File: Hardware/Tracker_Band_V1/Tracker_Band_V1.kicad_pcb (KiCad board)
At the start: 4 copper layers, 19.2 x 25.9 mm, 78 parts, among them J1 USB_C_USB20, Q1 SSM6L56FE, SW1 EVP-AVAA1A, SW2 EVP-AVAA1A, U1 ESP32-C3-MINI-1-N4, U2 BNO085, U3 RT8010, U4 MCP73832-2-AC, U5 LM66200, U6 IN-PI15TAT5R5G5B, U7 IN-PI15TAT5R5G5B, U8 IN-PI15TAT5R5G5B, U9 IN-PI15TAT5R5G5B, X1 32.768kHz

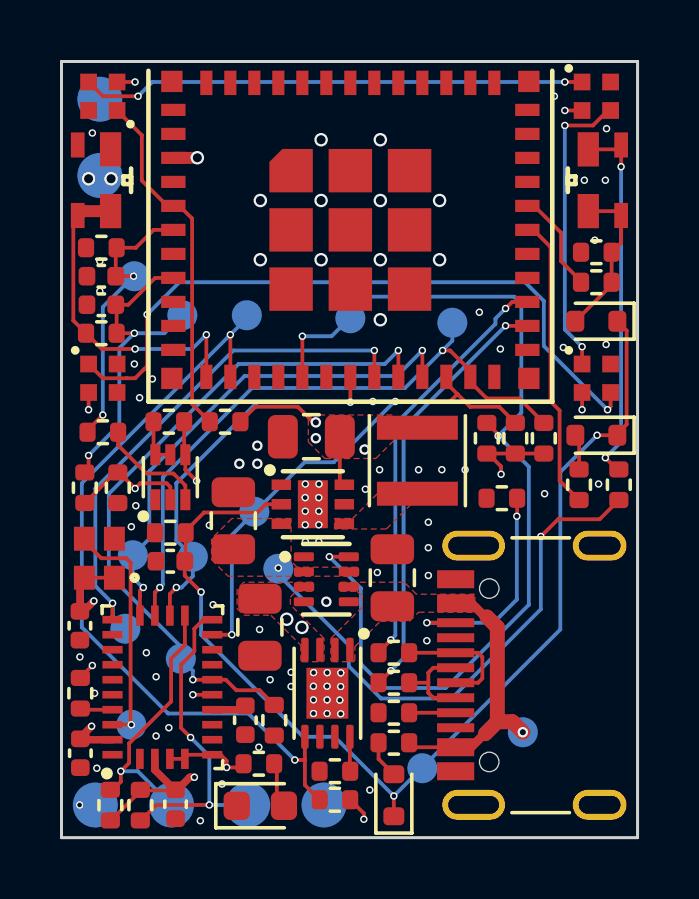
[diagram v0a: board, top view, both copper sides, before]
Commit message: SCH & PCB Finalized for review
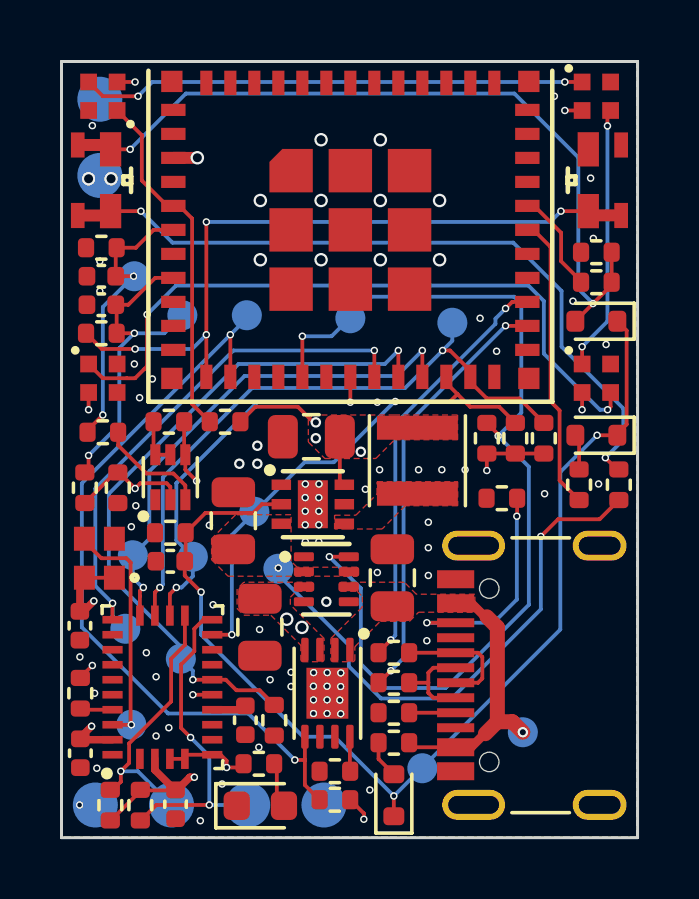
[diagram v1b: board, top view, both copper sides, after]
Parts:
- R19: value 10k -> 100k
- moved SW1 17.8 mm to (122.8, 79.5), turned to -90 degrees
- moved SW2 17.8 mm to (140.6, 79.5), turned to 90 degrees
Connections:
- SW2 pad 1: GND -> /SW_2
- SW2 pad 2: GND -> /SW_2
- SW2 pad 3: /SW_2 -> GND
- SW2 pad 4: /SW_2 -> GND
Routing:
- net /BUCK_EN_SW: track 5.31 -> 26.3 mm, vias 0 -> 2
- net /SW_2: track 11.1 -> 23.6 mm, vias 2 -> 4
- net Net-(SW1-A): track 12.4 -> 24.6 mm
- net /RGB_LED2: track 9.92 -> 8.90 mm
- net GND: vias 84 -> 81
- added copper zone on In2.Cu, net GND
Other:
- board text removed: "AN"
